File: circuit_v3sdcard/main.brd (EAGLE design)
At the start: 21.7 x 29.5 mm, 20 parts, among them CN1 SD, CN3 MICROSD, CN4 5035481020, IC1 C8051F381-GM, IC3 N25Q512A, IC4 KC2016K, IC6 MPU-9250

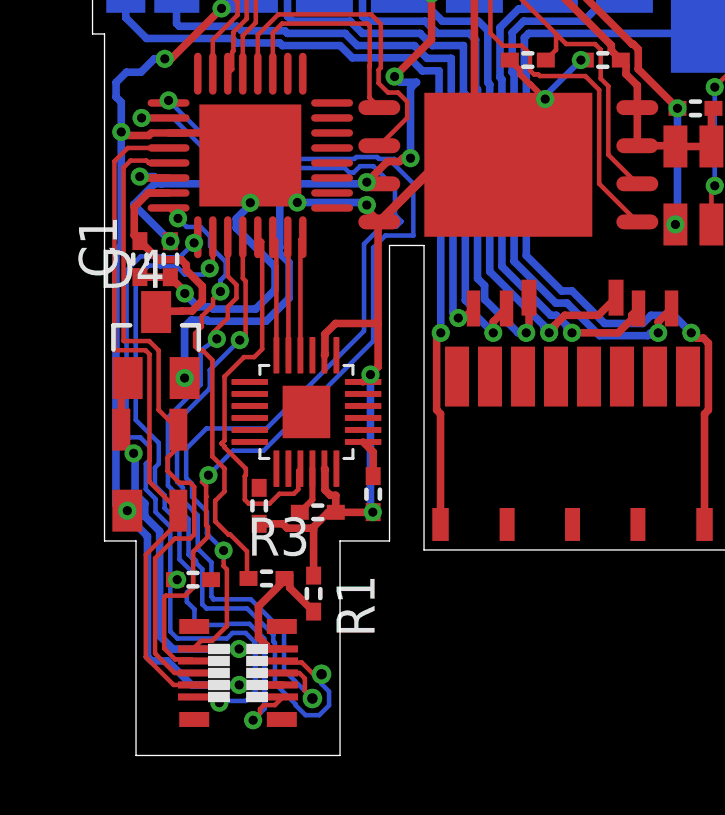
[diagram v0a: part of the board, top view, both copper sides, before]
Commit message: Modified circuit
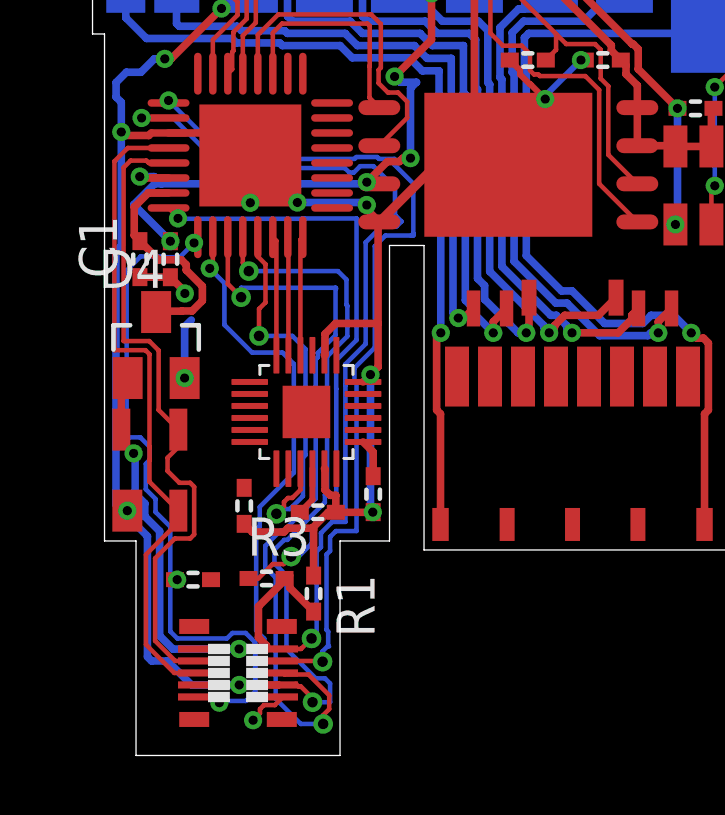
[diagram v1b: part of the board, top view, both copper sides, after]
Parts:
- moved C2 0.50 mm to (4.75, 8.42)
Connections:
- net D+: now also CN4.5; no longer CN4.7
- net D-: now also CN4.3; no longer CN4.5
- net DGND: now also CN4.7; no longer CN4.8
- net GPIO0: now also CN4.8; no longer CN4.6
- net GPIO1: now also CN4.6; no longer CN4.4
- net RX1: now also CN4.4; no longer CN4.3
- net TX1: now also CN4.2; no longer CN4.1
- net VBUS: now also CN4.1; no longer CN4.2
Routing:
- net +3V3: track 69.5 -> 61.9 mm
- net DGND: track 135.0 -> 128.3 mm
- net C2D: track 23.4 -> 17.4 mm
- net N$4: track 14.9 -> 20.6 mm
- net TX1: track 31.6 -> 28.5 mm
- net RX1: track 31.3 -> 29.3 mm
- net GPIO1: track 23.5 -> 25.4 mm
- net GPIO0: track 20.6 -> 22.2 mm
- net VBUS: track 18.1 -> 17.6 mm
- net IMU_MISO: track 12.7 -> 13.2 mm, vias 0 -> 2
